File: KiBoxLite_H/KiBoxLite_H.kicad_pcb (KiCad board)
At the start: 4 copper layers, 48.4 x 86.8 mm, 152 parts, among them J1 Screw_Terminal_01x03, J2 USB4105-GF-A-060, Q2 BC817-40(SOT23), Q3 BC817-40(SOT23), T1 LMUN2211LT1G(SOT-23), U1 CH340X(MSOP-10), U10 MAX13487, U3 TP4054-42-SOT25-R(SOT23-5), U4 LAN8710A-EZC(QFN32), U5 TX4138(ESOIC-8), U6 ESP32-WROOM-32E-N4, U7 TPS62A02ADRLR(SOT-563-6), U8 NA(SN74LVC1G04DBVR(SOT23-5)), U9 TPS2378DDAR(HSOIC-8)

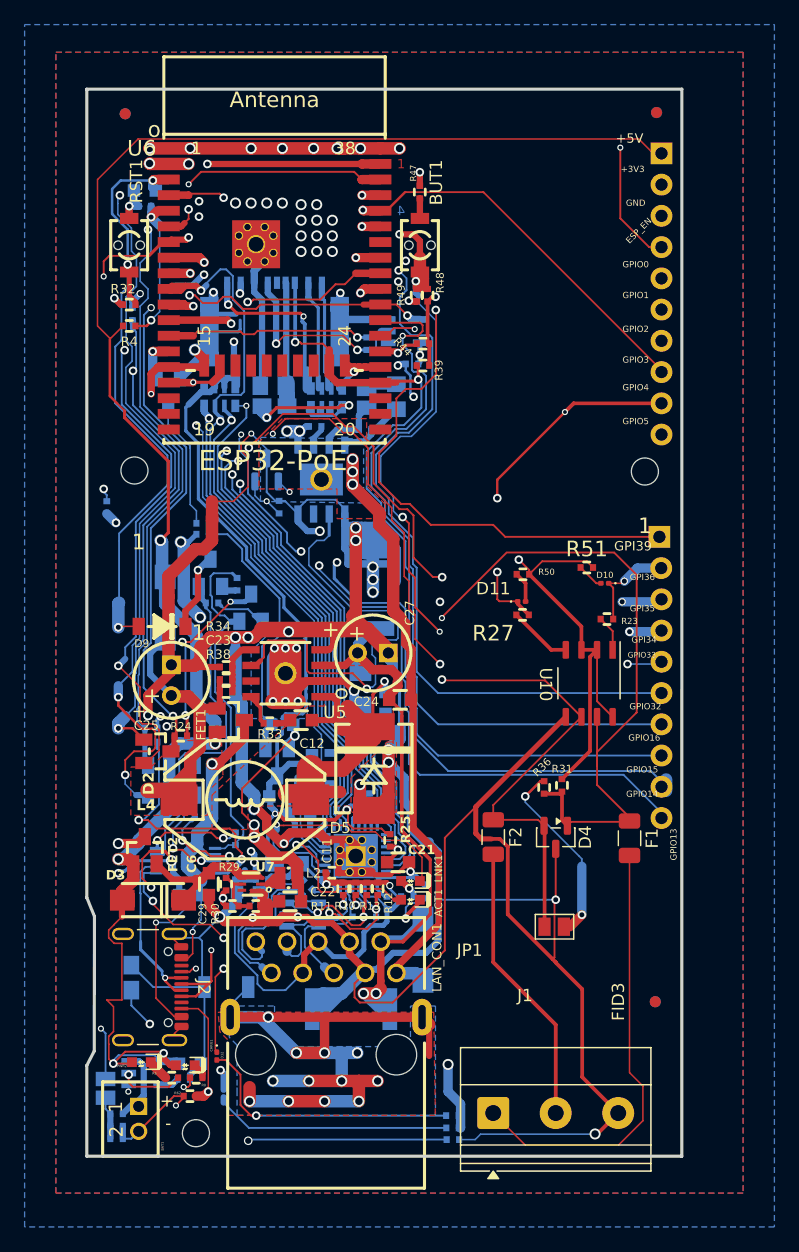
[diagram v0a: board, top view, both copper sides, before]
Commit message: build: 0 errores 2
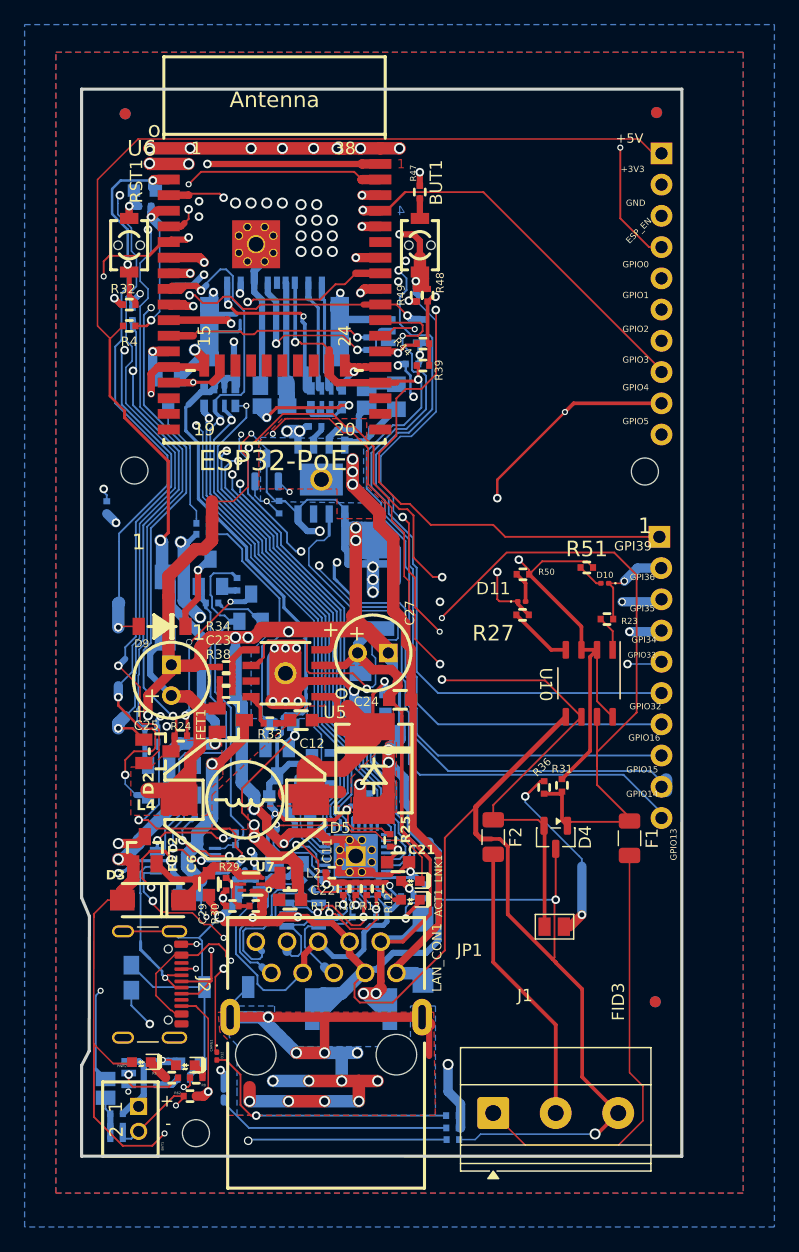
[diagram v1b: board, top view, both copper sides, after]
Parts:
- moved J2 0.21 mm to (92.9, 159.3)
- moved C22 0.13 mm to (105.4, 152.4)
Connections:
- FID4 pad e: unconnected-(FID4-FID*-PadFid1) -> (no net)
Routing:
- net +5V: track 227.8 -> 235.8 mm
- net GND: track 611.3 -> 614.3 mm, vias 63 -> 64
- net VBUS: track 38.7 -> 38.1 mm
- net Net-(Q3-C): track 15.1 -> 14.6 mm
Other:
- board size 48.4 x 86.8 mm -> 48.8 x 86.8 mm
